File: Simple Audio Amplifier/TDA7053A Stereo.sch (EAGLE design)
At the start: 23 parts, among them IC1 TDA7052A

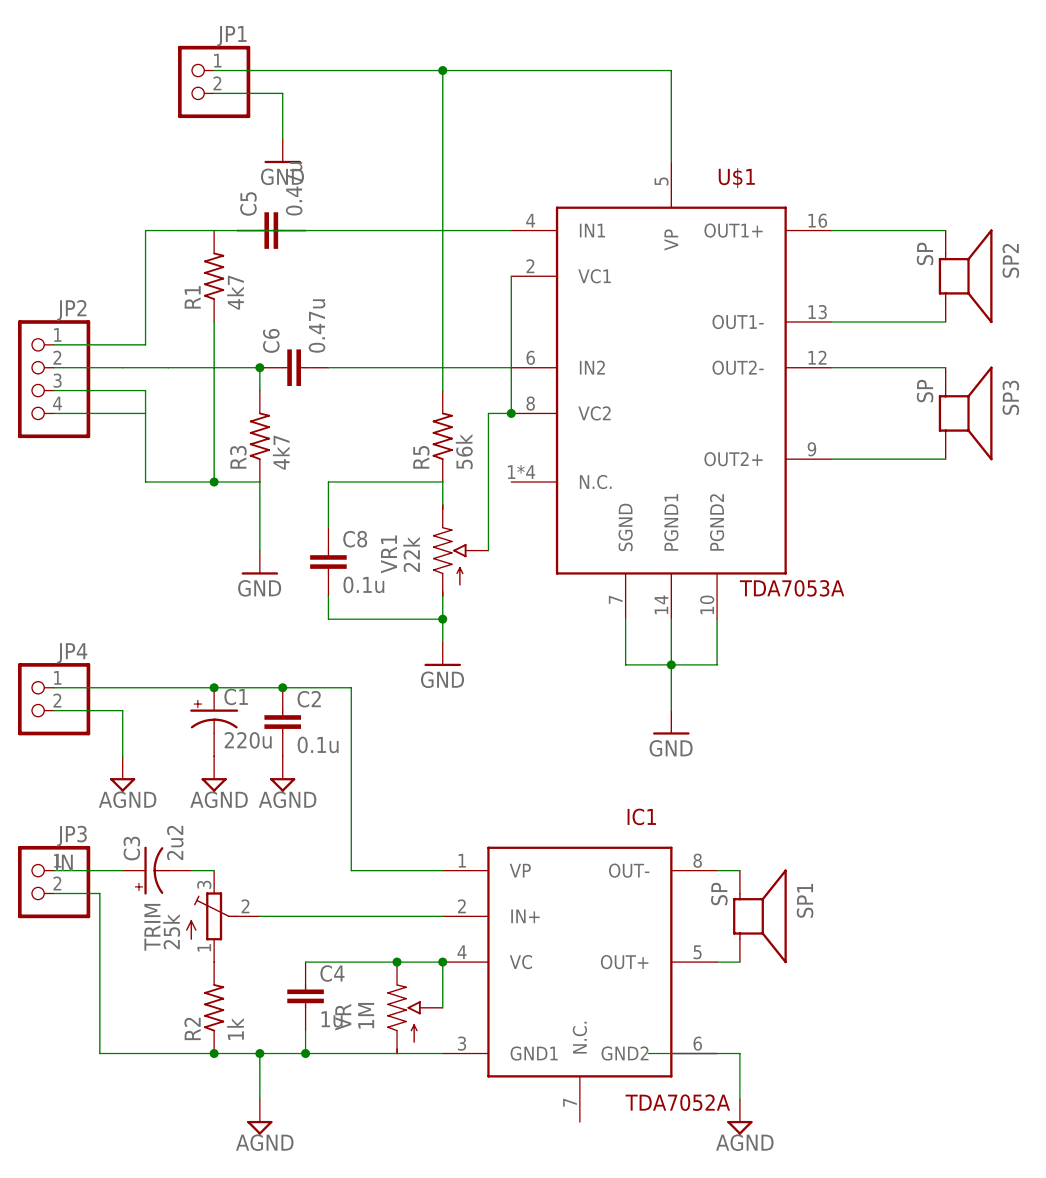
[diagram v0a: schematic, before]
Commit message: Simple Audio Amp
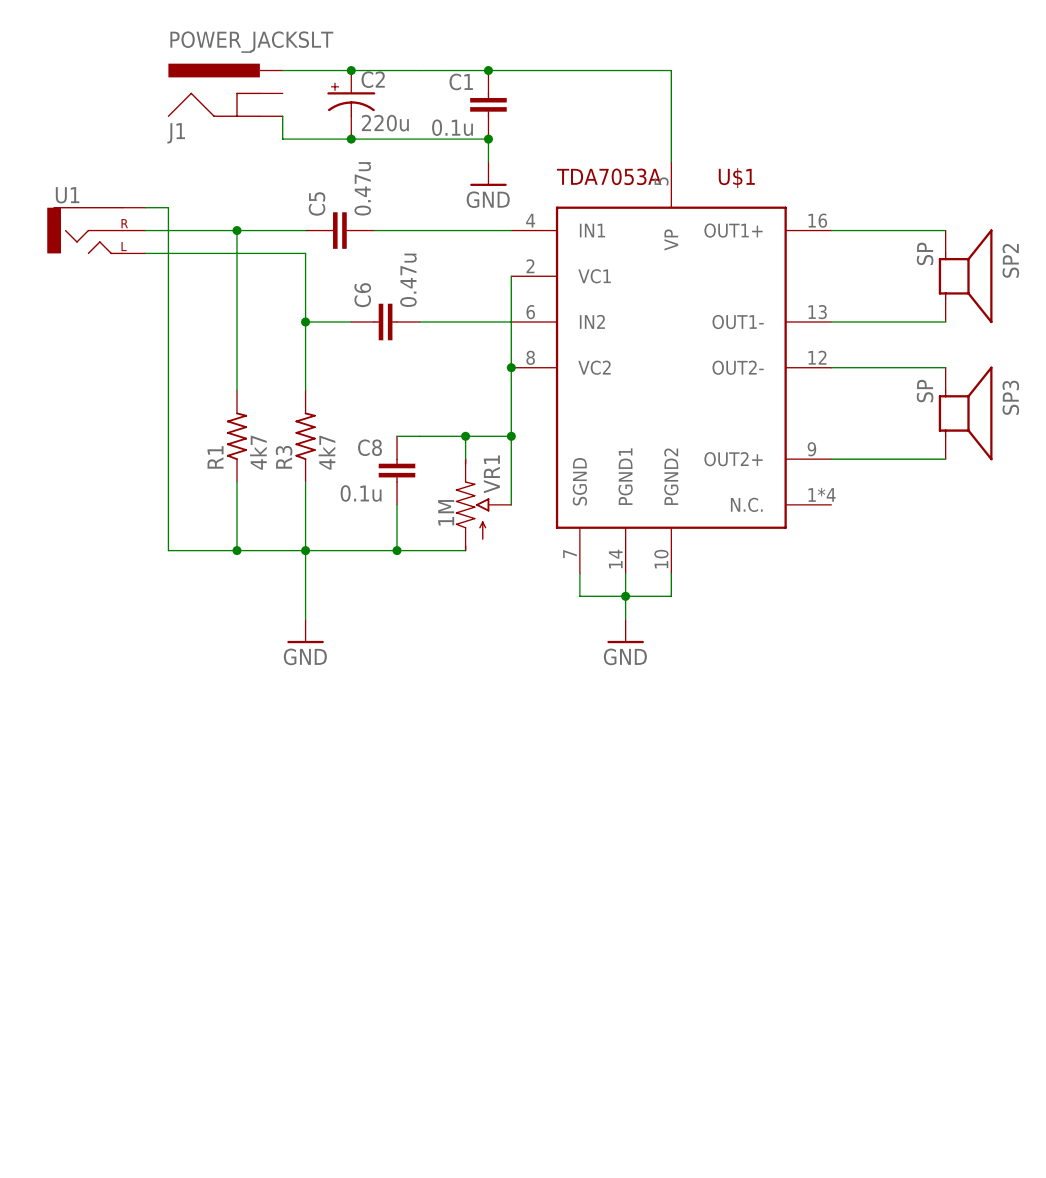
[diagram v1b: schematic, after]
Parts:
- removed C3: 2u2, SparkFun:CAP_POLPTH1
- removed C4: 1u, SparkFun:CAPPTH2
- removed IC1: TDA7052A, My Library:TDA7052A
- removed JP1, JP3, JP4: (no value), pinhead:PINHD-1X2
- removed JP2: (no value), pinhead:PINHD-1X4
- removed R2: 1k, adafruit:R-US_0204/5
- removed R5: 56k, adafruit:R-US_0204/5
- removed SP1: SP, My Library:SP
- removed TRIM: 25k, adafruit:TRIMPOTTC33X
- removed VR: 1M, My Library:POT-RV16AF-20
- added J1: POWER_JACKSLT, SparkFun:POWER_JACKSLT
- added U1: (no value), SparkFun:AUDIO-JACKPTH
- C1: value 220u -> 0.1u; device SparkFun:CAP_POLPTH1 -> SparkFun:CAPPTH2
- C2: value 0.1u -> 220u; device SparkFun:CAPPTH2 -> SparkFun:CAP_POLPTH1
- VR1: value 22k -> 1M
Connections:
- removed net AGND: C1.-, C2.2, C4.2, IC1.GND1, IC1.GND2, JP3.2, JP4.2, R2.1, VR.A
- removed net IN: C3.+, JP3.1
- removed net N$1: C1.+, C2.1, IC1.VP, JP4.1
- removed net N$13: C3.-, TRIM.E
- removed net N$16: C8.1, R5.1, VR1.E
- removed net N$2: IC1.IN+, TRIM.S
- removed net N$3: R2.2, TRIM.A
- removed net N$5: C4.1, IC1.VC, VR.E, VR.S
- removed net N$8: IC1.OUT-, SP1.+
- removed net N$9: IC1.OUT+, SP1.-
- net GND: now also C1.2, C2.-, J1.GND, U1.SLEEVE; no longer JP1.2, JP2.3, JP2.4
- net N$17: now also C1.1, C2.+, J1.PWR; no longer JP1.1, R5.2
- net N$19: now also C8.1, VR1.E
- net N$4: now also U1.RIGHT; no longer JP2.1
- net N$6: now also U1.LEFT; no longer JP2.2
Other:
- moved on the sheet: C5, C6, C8, R1, R3, U$1, VR1
